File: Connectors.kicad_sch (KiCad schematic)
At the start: 10 parts, among them J701 1-00777, J702 ESMC-F-80-SGS-SMT-A-PP-T_R, U701 ${MANUFACTURER PART NUMBER}, U702 PCA9675PW,118, U703 ${MANUFACTURER PART NUMBER}

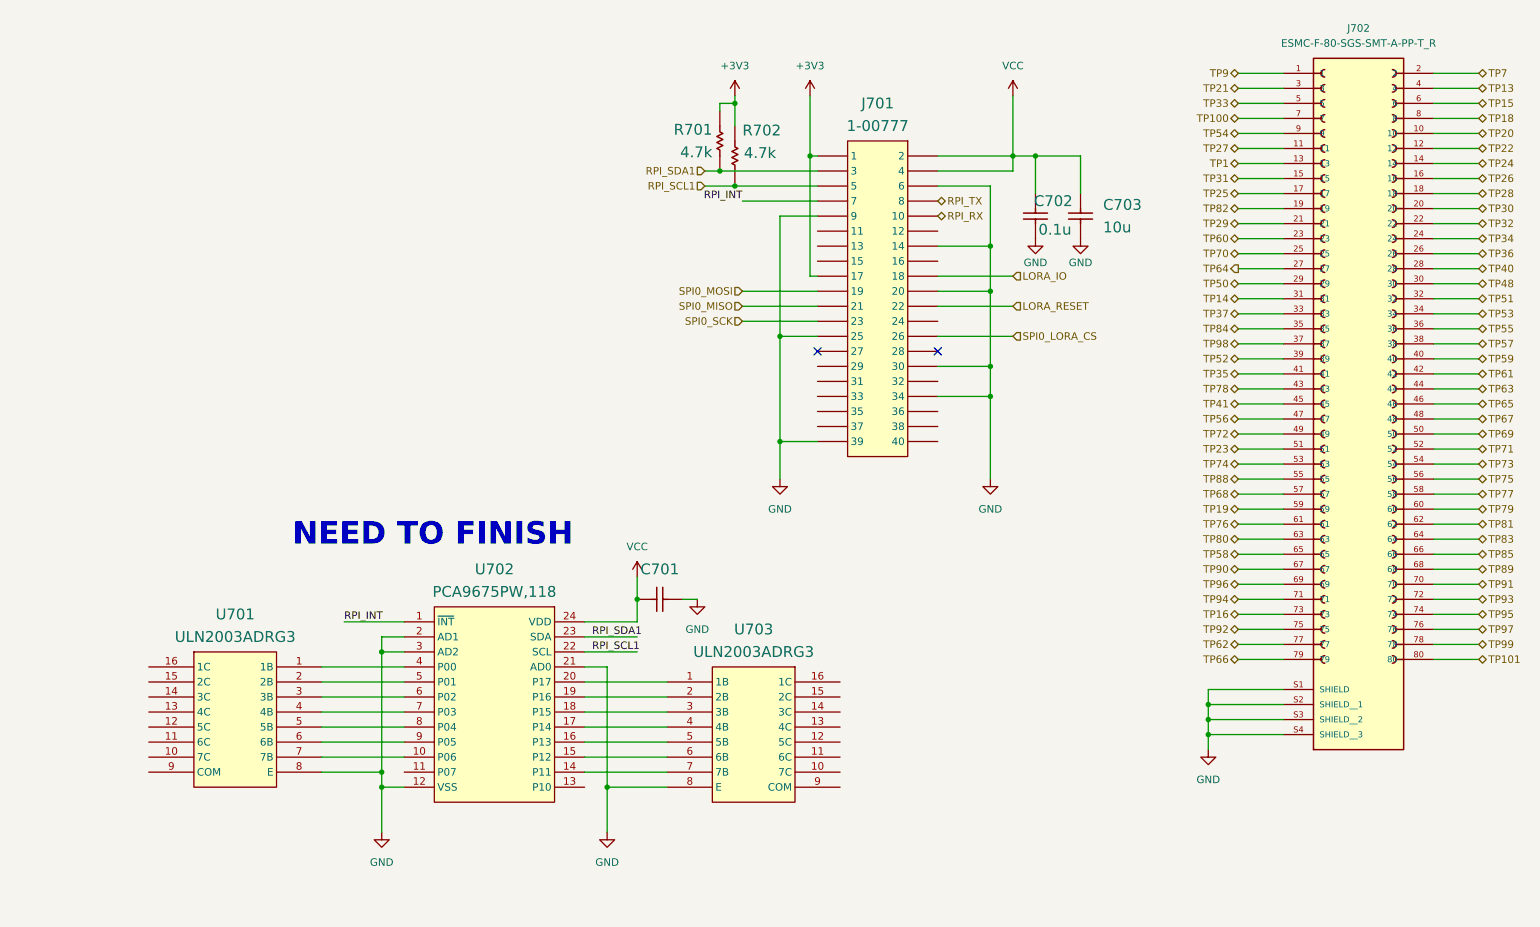
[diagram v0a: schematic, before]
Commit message: V0.1 for review
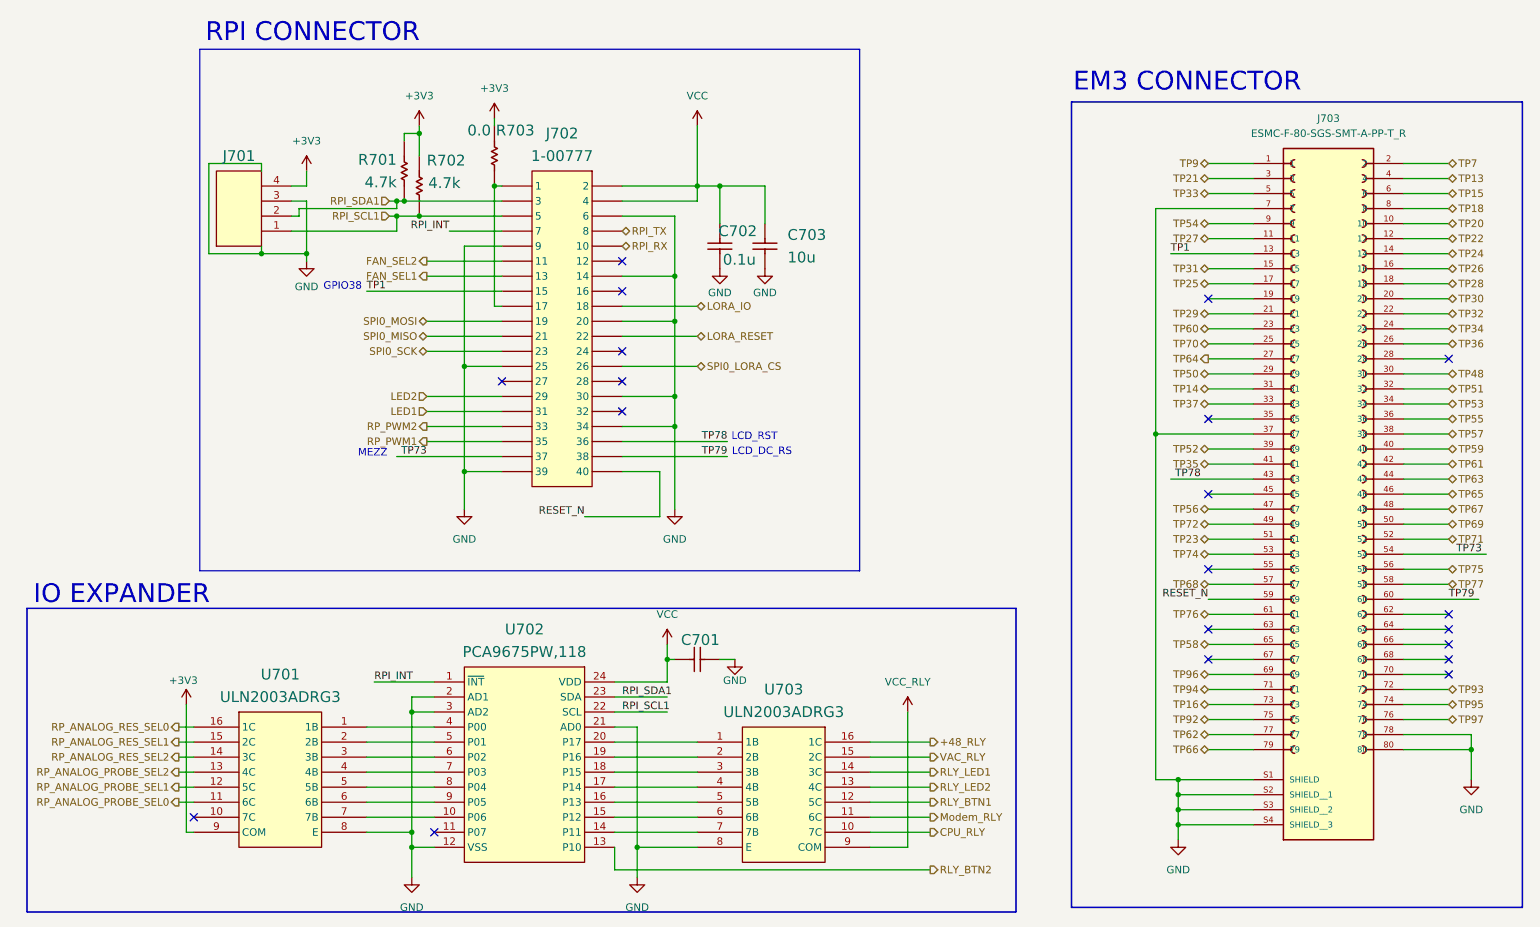
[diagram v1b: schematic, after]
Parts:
- added J701: 1-00837, CONN:JST_BM04B-SRSS-TB(LF)(SN), symbol EXACT_CONN:1-00837
- added R703: ${VALUE}, RES:RES_0603, symbol EXACT_RES:1-00015
- C701, R701: value ${VALUE} -> ~
- renumbered J701 to J702, J702 to J703
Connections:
- net TP100 is gone; now on net GND: J703.7
- net TP101 is gone; now on net GND: J703.80
- net TP19 is gone; now on net RESET_N: J703.59
- net TP98 is gone; now on net GND: J703.37
- net TP99 is gone; now on net GND: J703.78
- net +3V3: now also U701.9 (COM), J701.4, R703.1; no longer J702.1, J702.17
- net GND: now also J701.3, J701.S1, J701.S2
- net RPI_SCL1: now also J701.1
- net RPI_SDA1: now also J701.2
- net TP1: now also J702.15
- net TP73: now also J702.37
- net TP78: now also J702.36
- net TP79: now also J702.38
- net RP_ANALOG_PROBE_SEL0: now reaches U701.11 (6C)
- net RP_ANALOG_PROBE_SEL1: now reaches U701.12 (5C)
- net RP_ANALOG_PROBE_SEL2: now reaches U701.13 (4C)
- net RP_ANALOG_RES_SEL2: now reaches U701.14 (3C)
- net RP_ANALOG_RES_SEL1: now reaches U701.15 (2C)
- net RP_ANALOG_RES_SEL0: now reaches U701.16 (1C)
- net FAN_SEL2: now reaches J702.11
- net FAN_SEL1: now reaches J702.13
- net LED2: now reaches J702.29
- net LED1: now reaches J702.31
- net RP_PWM2: now reaches J702.33
- net RP_PWM1: now reaches J702.35
- net RESET_N: now reaches J702.40
- net RLY_BTN2: now reaches U702.13 (P10)
- net CPU_RLY: now reaches U703.10 (7C)
- net Modem_RLY: now reaches U703.11 (6C)
- net RLY_BTN1: now reaches U703.12 (5C)
- net RLY_LED2: now reaches U703.13 (4C)
- net RLY_LED1: now reaches U703.14 (3C)
- net VAC_RLY: now reaches U703.15 (2C)
- net +48_RLY: now reaches U703.16 (1C)
- net VCC_RLY: now reaches U703.9 (COM)
- net TP40: no longer names the net of J703.28
- net TP41: no longer names the net of J703.45
- net TP80: no longer names the net of J703.63
- net TP81: no longer names the net of J703.62
- net TP82: no longer names the net of J703.19
- net TP83: no longer names the net of J703.64
- net TP84: no longer names the net of J703.35
- net TP85: no longer names the net of J703.66
- net TP88: no longer names the net of J703.55
- net TP89: no longer names the net of J703.68
- net TP90: no longer names the net of J703.67
- net TP91: no longer names the net of J703.70
- new net: J702.1, J702.17, R703.2
- no-connect marks 2 -> 20
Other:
- note added: "EM3 CONNECTOR"
- note added: "GPIO38"
- note added: "IO EXPANDER"
- note added: "LCD_DC_RS"
- note added: "LCD_RST"
- note added: "MEZZ"
- note added: "RPI CONNECTOR"
- note removed: "NEED TO FINISH"
- moved on the sheet: C701, C702, C703, J702, J703, R701, R702, U701, U702, U703
